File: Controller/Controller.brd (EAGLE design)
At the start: 100 x 80 mm, 7 parts, among them U1 TPD4S009DBVR, U2 TPS2511DGN

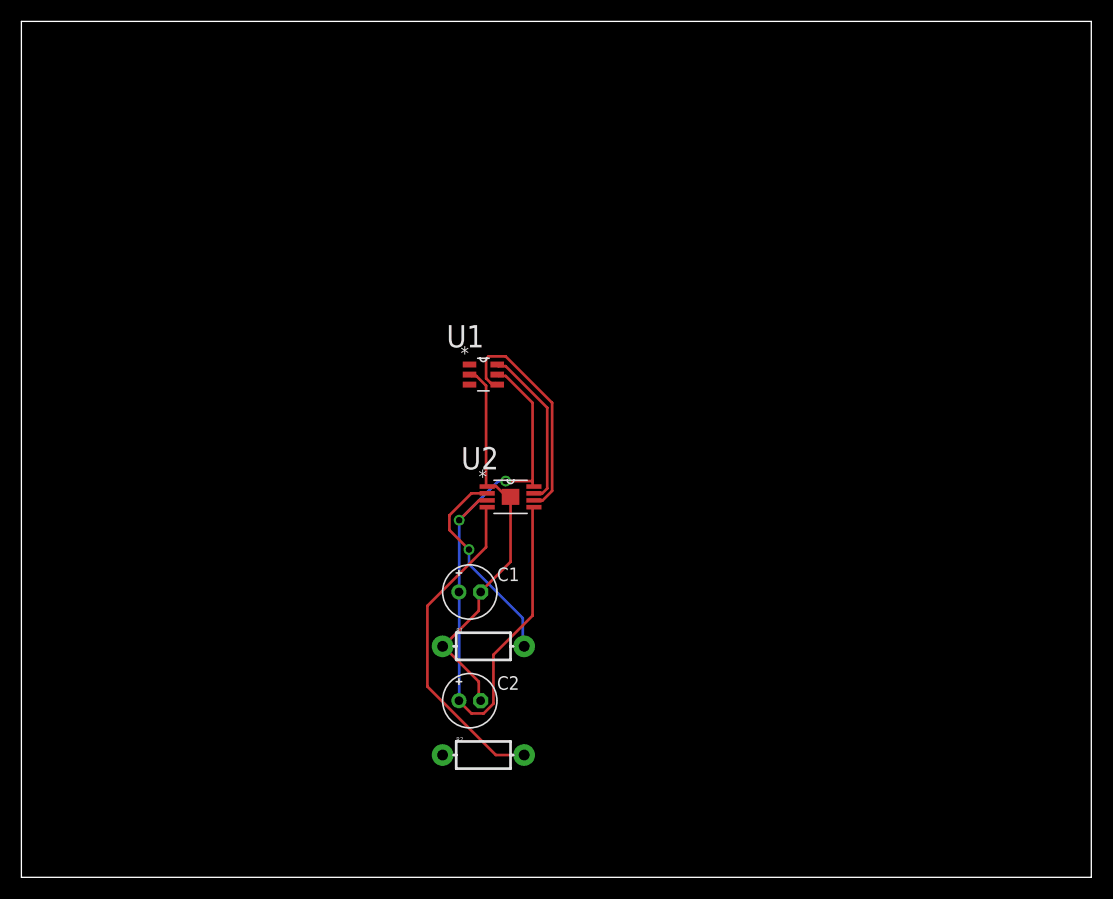
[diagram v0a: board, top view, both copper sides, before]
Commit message: Modified controller
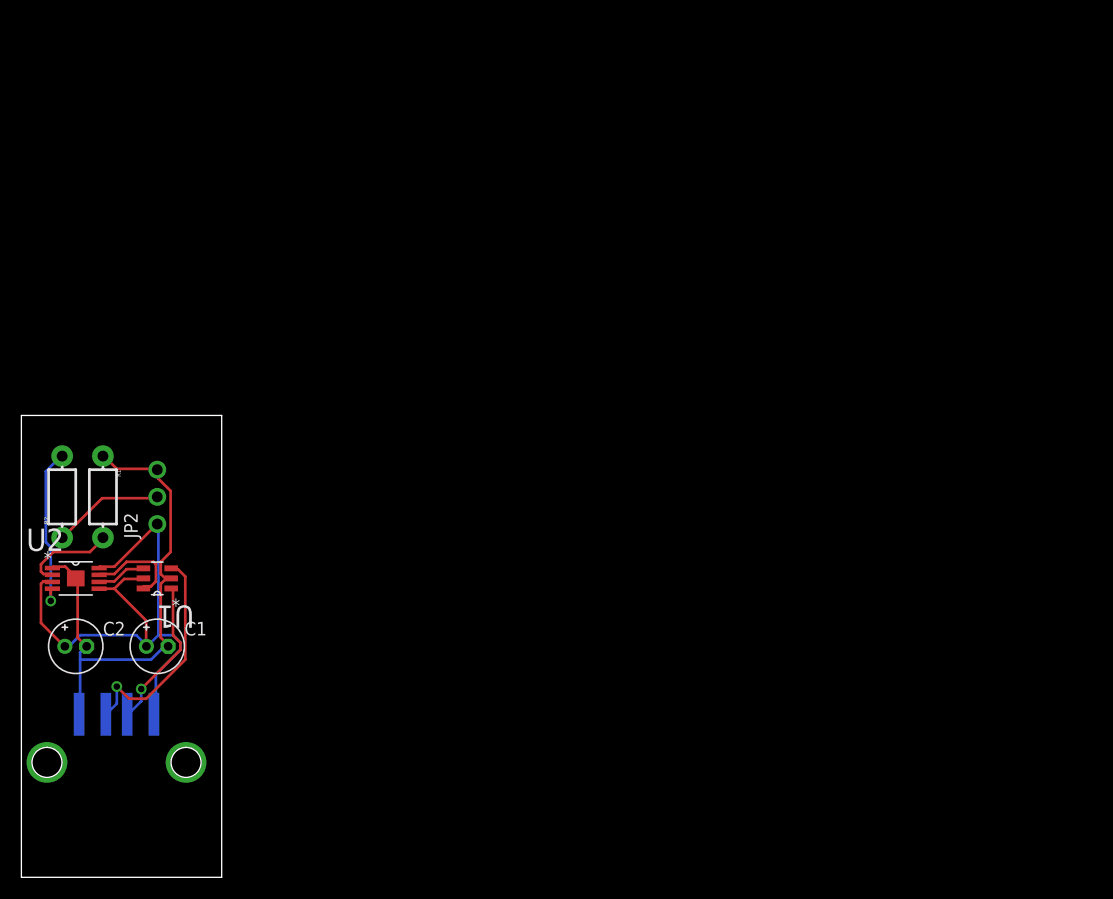
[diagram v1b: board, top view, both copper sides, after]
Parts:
- added JP2: (no value), adafruit:1X03-CLEANBIG
- added U$1: SPARKFUN_USB_A, sparkfun-usb-a:USB_4UCON_18666_318
- moved R2 46.2 mm to (3.81, 35.6), turned to 90 degrees
- moved U2 41.3 mm to (5.08, 27.9)
- moved R1 38.2 mm to (7.62, 35.6), turned to 270 degrees
- moved C2 37.2 mm to (5.08, 21.6)
- moved U1 35.9 mm to (12.7, 27.9), turned to 180 degrees
- moved C1 29.6 mm to (12.7, 21.6)
- moved FRAME1 11.5 mm to (33.0, -8.89)
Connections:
- new net N$9: JP2.2, R2.P$1
- net N$1: now also U$1.USB+
- net N$2: now also U$1.USB-
- net N$3: now also JP2.1, U$1.USB_5V
- net N$4: now also JP2.3, U$1.USB_GND
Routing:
- net N$1: track 0.00 -> 20.8 mm, vias 0 -> 1
- net N$6: track 21.5 -> 4.65 mm
- net N$8: track 30.8 -> 15.7 mm, vias 0 -> 1
- net N$2: track 0.00 -> 14.3 mm, vias 0 -> 1
- net N$4: track 37.3 -> 49.8 mm
- net N$7: track 19.5 -> 8.74 mm, vias 1 -> 0
- net N$9: track 0.00 -> 10.5 mm
- net N$3: track 65.0 -> 56.9 mm, vias 2 -> 0
- net N$5: track 15.3 -> 9.05 mm
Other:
- board size 100 x 80 mm -> 18.7 x 43.2 mm
